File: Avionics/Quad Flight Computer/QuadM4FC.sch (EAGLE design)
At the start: 7 parts, among them U1 INF-PG-LQFP-100-11-7000X7000E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, U2 MPU-9250, U3 MPL115A2, U4 S25FL127S, U5 CC2520, U6 CC2592, U7 CC1120

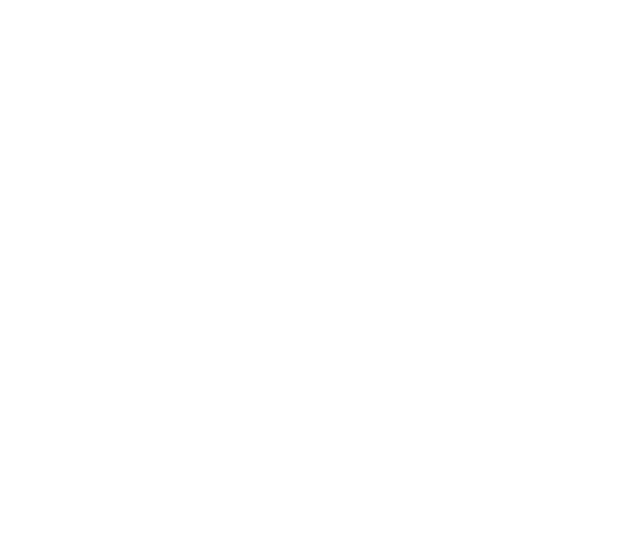
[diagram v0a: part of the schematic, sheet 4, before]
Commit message: Added RF base station project
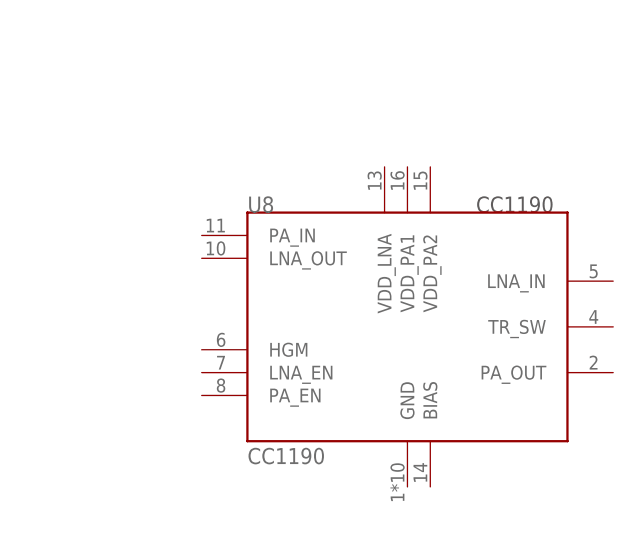
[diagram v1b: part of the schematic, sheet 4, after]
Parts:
- added U8: CC1190, ti_rf:CC1190
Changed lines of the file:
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@@
 <part name="U6" library="ti_rf" deviceset="CC2592" device=""/>
 <part name="U7" library="ti_rf" deviceset="CC1120" device=""/>
+<part name="U8" library="ti_rf" deviceset="CC1190" device=""/>
 </parts>
 <sheets>
@@
 <instances>
 <instance part="U7" gate="G$1" x="0" y="0"/>
+<instance part="U8" gate="G$1" x="93.98" y="-10.16"/>
 </instances>
 <busses>
